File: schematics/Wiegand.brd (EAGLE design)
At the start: 79 x 58.2 mm, 83 parts, among them J1 AVR_SPI_PRG_6NS, U1 ATMEGA168, U2 RS485_SP491, U3 MIC5219 5V, U4 MOC3063, U5 MOC3063, U6 MOC3063, U7 MOC3063, U8 MOC3063, U9 MOC3063, X1 RJ45-8PTH, X2 RJ45-8PTH, Y1 16Mhz

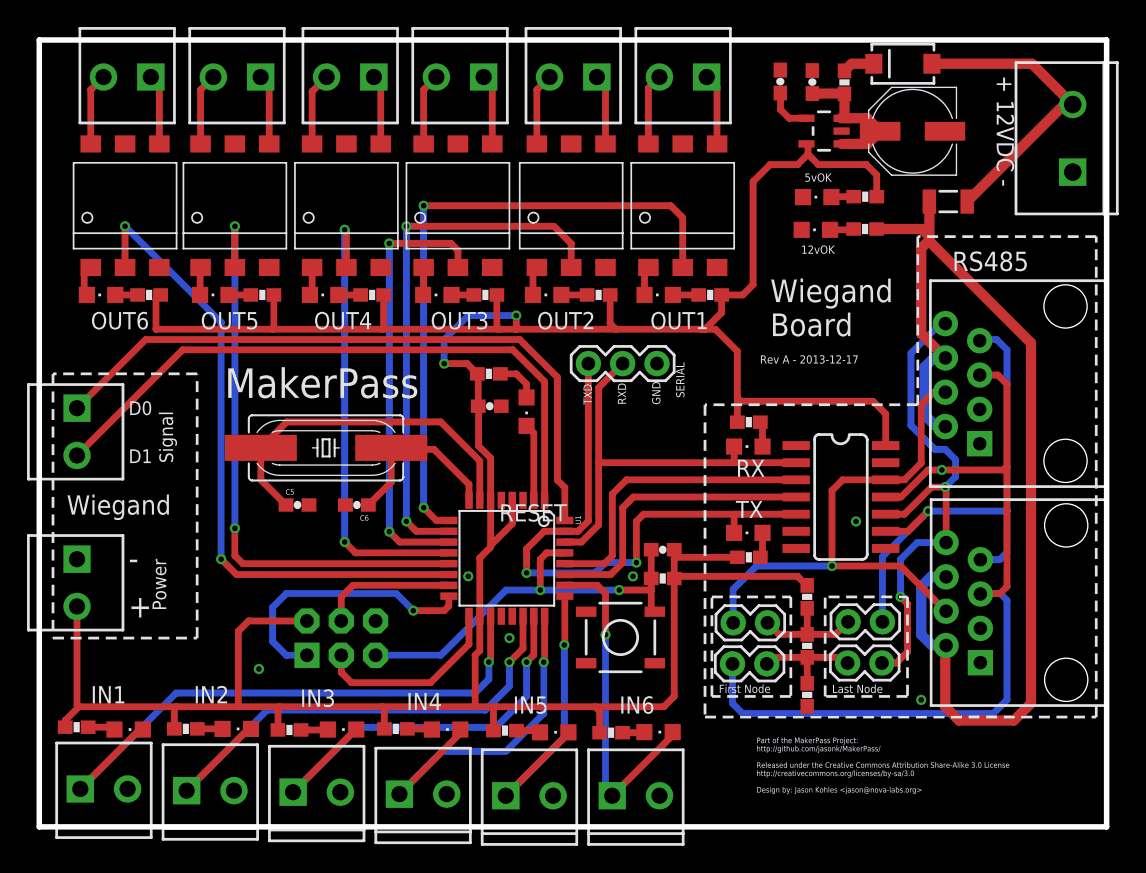
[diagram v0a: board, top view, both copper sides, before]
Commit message: Board Rev B
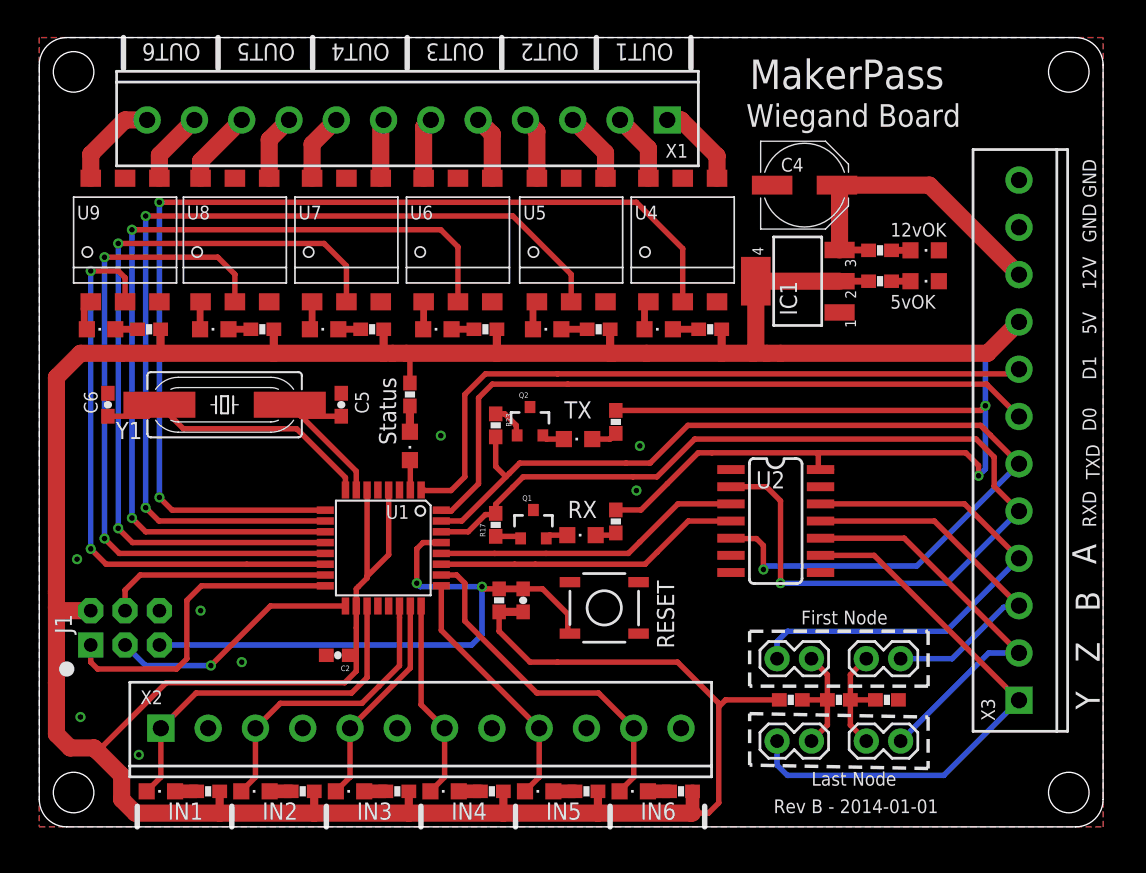
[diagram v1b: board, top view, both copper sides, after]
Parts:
- removed C1: 2.2uF Tantalum, SparkFun-Capacitors:0603-CAP
- removed C3: 0.1uF 50V, SparkFun-Capacitors:0603-CAP
- removed D1: (no value), SparkFun:SMA-DIODE
- removed F1: PTCSMD, SparkFun:PTC-1206
- removed JP1: 12VDC, SparkFun:SCREWTERMINAL-5MM-2
- removed JP10: INPUT5, SparkFun:SCREWTERMINAL-3.5MM-2
- removed JP11: INPUT6, SparkFun:SCREWTERMINAL-3.5MM-2
- removed JP12: OUTPUT1, SparkFun:SCREWTERMINAL-3.5MM-2
- removed JP13: OUTPUT2, SparkFun:SCREWTERMINAL-3.5MM-2
- removed JP14: OUTPUT3, SparkFun:SCREWTERMINAL-3.5MM-2
- removed JP15: OUTPUT4, SparkFun:SCREWTERMINAL-3.5MM-2
- removed JP16: OUTPUT5, SparkFun:SCREWTERMINAL-3.5MM-2
- removed JP17: OUTPUT6, SparkFun:SCREWTERMINAL-3.5MM-2
- removed JP18: Wiegand-Signal, SparkFun:SCREWTERMINAL-3.5MM-2
- removed JP19: Wiegand-Power, SparkFun:SCREWTERMINAL-3.5MM-2
- removed JP21: SERIAL, SparkFun-Connectors:1X03
- removed JP6: INPUT3, SparkFun:SCREWTERMINAL-3.5MM-2
- removed JP7: INPUT4, SparkFun:SCREWTERMINAL-3.5MM-2
- removed JP8: INPUT1, SparkFun:SCREWTERMINAL-3.5MM-2
- removed JP9: INPUT2, SparkFun:SCREWTERMINAL-3.5MM-2
- removed U3: MIC5219 5V, SparkFun-PowerIC:SOT23-5
- added IC1: (no value), linear:SOT223
- added Q1, Q2: NTR1P02T1G, SparkFun:SOT23-3
- added R23: 10K, SparkFun:0603-RES
- added X3: (no value), LumisenseV6:CON-1X12-TERMBLOCK-3.5MM
- C2: value 470pF -> 100nF; device SparkFun-Capacitors:0603-CAP -> SparkFun:0603-CAP
- C4: value 220uF 35V -> 47uF; device SparkFun-Capacitors:PANASONIC_D -> rcl:PANASONIC_D
- JP2: value First Node -> First Node A
- JP3: value Last Node -> Last Node Y
- JP4: value First Node -> First Node B
- JP5: value Last Node -> Last Node Z
- LED1: value 5V OK -> GRN
- LED10: value INPUT6 -> RED
- LED11: value OUTPUT2 -> RED
- LED12: value OUTPUT1 -> RED
- LED13: value OUTPUT3 -> RED
- LED14: value OUTPUT4 -> RED
- LED15: value OUTPUT5 -> RED
- LED16: value OUTPUT6 -> RED
- LED17: value STATUS -> YLW
- LED2: value RX -> RED
- LED3: value TX -> RED
- LED4: value 12V OK -> GRN
- LED5: value INPUT3 -> RED
- LED6: value INPUT4 -> RED
- LED7: value INPUT1 -> RED
- LED8: value INPUT2 -> RED
- LED9: value INPUT5 -> RED
- R17: value 12 ohm 5 watt -> 10K
- X1, X2: value RJ45-8PTH -> (none); device SparkFun:RJ45-8 -> LumisenseV6:CON-1X12-TERMBLOCK-3.5MM
- moved X2 71.6 mm to (9.00, 7.30), turned to 0 degrees
- moved C2 53.6 mm to (22.1, 12.7), turned to 180 degrees
- moved U$4 47.5 mm to (26.9, 51.1), turned to 270 degrees
- moved X1 46.3 mm to (46.5, 52.3), turned to 180 degrees
- moved R17 41.7 mm to (33.8, 22.4), turned to 90 degrees
- moved C6 19.9 mm to (5.08, 31.2), turned to 90 degrees
- moved J1 16.0 mm to (6.35, 14.7)
- moved LED2 12.6 mm to (39.9, 28.7)
- moved JP4 12.5 mm to (63.8, 12.4), turned to 180 degrees
- moved LED3 12.3 mm to (40.1, 21.6)
- moved R1 12.2 mm to (34.0, 16.8), turned to 270 degrees
- moved C7 11.0 mm to (35.8, 16.8), turned to 90 degrees
- moved R4 10.8 mm to (12.5, 2.63), turned to 0 degrees
- moved R10 10.2 mm to (42.7, 22.6), turned to 90 degrees
- moved LED1 10.1 mm to (65.5, 40.4), turned to 270 degrees
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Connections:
- removed net 12V_IN: D1.A, F1.1, JP1.2
- new net N$42: Q2.1, R23.1
- net +12V: now also C4.+, IC1.3, X3.10; no longer F1.2, X1.2, X1.6, X2.2, X2.6
- net D0: now also X3.7; no longer JP18.1
- net D1: now also X3.8; no longer JP18.2
- net GND: now also IC1.1, Q1.3, Q2.3, X2.10, X2.12, X2.2, X2.4, X2.6, X2.8, X3.11, X3.12; no longer C1.2, C3.2, JP1.1, JP10.2, JP11.2, JP19.1, JP21.1, JP6.2, JP7.2, JP8.2, JP9.2, U3.2, X1.1, X1.3, X2.1, X2.3
- net INPUT1: now also X2.1; no longer JP8.1
- net INPUT2: now also X2.3; no longer JP9.1
- net INPUT3: now also X2.5; no longer JP6.1
- net INPUT4: now also X2.7; no longer JP7.1
- net INPUT5: now also X2.9; no longer JP10.1
- net INPUT6: now also X2.11; no longer JP11.1
- net N$17: now also X1.1; no longer JP12.1
- net N$18: now also X1.2; no longer JP12.2
- net N$19: now also X1.3; no longer JP13.1
- net N$20: now also X1.4; no longer JP13.2
- net N$23: now also X1.5; no longer JP14.1
- net N$24: now also X1.6; no longer JP14.2
- net N$29: now also X1.7; no longer JP15.1
- net N$3: now also U8.4, X1.9; no longer C2.1, U3.4
- net N$30: now also X1.8; no longer JP15.2
- net N$33: now also LED2.C, Q2.2; no longer JP16.1, U8.4
- net N$34: now also Q1.1, R17.1; no longer JP16.2, U8.6
- net N$37: now also X1.11; no longer JP17.1
- net N$38: now also X1.12; no longer JP17.2
- net N$4: now also U8.6, X1.10; no longer C3.1, C4.+, R17.2, U3.1, U3.3
- net N$9: now also LED3.C, Q1.2; no longer D1.C, R17.1
- net RS485-A: now also X3.4; no longer X1.4, X2.4
- net RS485-B: now also X3.3; no longer X1.5, X2.5
- net RS485-Y: now also X3.1; no longer X1.7, X2.7
- net RS485-Z: now also X3.2; no longer X1.8, X2.8
- net RXD: now also R17.2, X3.5; no longer JP21.2, LED2.C
- net TXD: now also R23.2, X3.6; no longer JP21.3, LED3.C
- net VCC: now also C2.1, IC1.2, IC1.4, X3.9; no longer C1.1, JP19.2, U3.5
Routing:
- net VCC: track 243.1 -> 342.5 mm
- net +12V: track 81.1 -> 23.4 mm
- net RXD: track 31.6 -> 79.5 mm, vias 0 -> 1
- net RS485-B: track 62.9 -> 27.7 mm, vias 1 -> 0
- net TXD: track 43.8 -> 78.2 mm, vias 2 -> 1
- net OUTPUT3: track 32.6 -> 64.8 mm
- net OUTPUT2: track 39.8 -> 70.6 mm
- net OUTPUT1: track 47.8 -> 78.6 mm
- net OUTPUT4: track 34.0 -> 57.1 mm
- net 12V_IN: track 22.5 -> 0.00 mm
- net INPUT1: track 44.8 -> 27.2 mm, vias 1 -> 0
- net INPUT2: track 39.3 -> 22.1 mm, vias 1 -> 0
- net INPUT3: track 33.0 -> 16.0 mm, vias 1 -> 0
- net RESET: track 31.4 -> 45.9 mm
- net N$100: track 26.1 -> 12.5 mm
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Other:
- board size 79 x 58.2 mm -> 78.7 x 58.4 mm
- board text added: "12V"
- board text added: "5V"
- board text added: "A"
- board text added: "B"
- board text added: "Design by: Jason Kohles <jason@nova-labs.org> Ted Markson <ted@nova-labs.org>"
- board text added: "Part of the MakerPass Project: http://github.com/jasonk/MakerPass/ Released under the Creative Commons Attribution Share-Alike 3.0 License http://creativecommons.org/licenses/by-sa/3.0"
- board text added: "Rev B - 2014-01-01"
- board text added: "Status"
- board text added: "Y"
- board text added: "Z"
- board text removed: "+"
- board text removed: "+ 12VDC -"
- board text removed: "-"
- board text removed: "Part of the MakerPass Project: http://github.com/jasonk/MakerPass/ Released under the Creative Commons Attribution Share-Alike 3.0 License http://creativecommons.org/licenses/by-sa/3.0 Design by: Jason Kohles <jason@nova-labs.org>"
- board text removed: "Power"
- board text removed: "RS485"
- board text removed: "Rev A - 2013-12-17"
- board text removed: "SERIAL"
- board text removed: "Signal"
- board text removed: "Wiegand"
